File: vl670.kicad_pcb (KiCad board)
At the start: 4 copper layers, 60.3 x 22.4 mm, 72 parts, among them J1 Conn_01x07_Male, J2 USB_C_Receptacle, J3 Conn_01x07_Male, J4 USB3_A Receptacle, J5 Conn_01x02_Male, U1 HD3SS3220, U2 VL670, U3 4016, U4 TPS2061C-PXLI, U6 GD25D05, Y1 25MHz

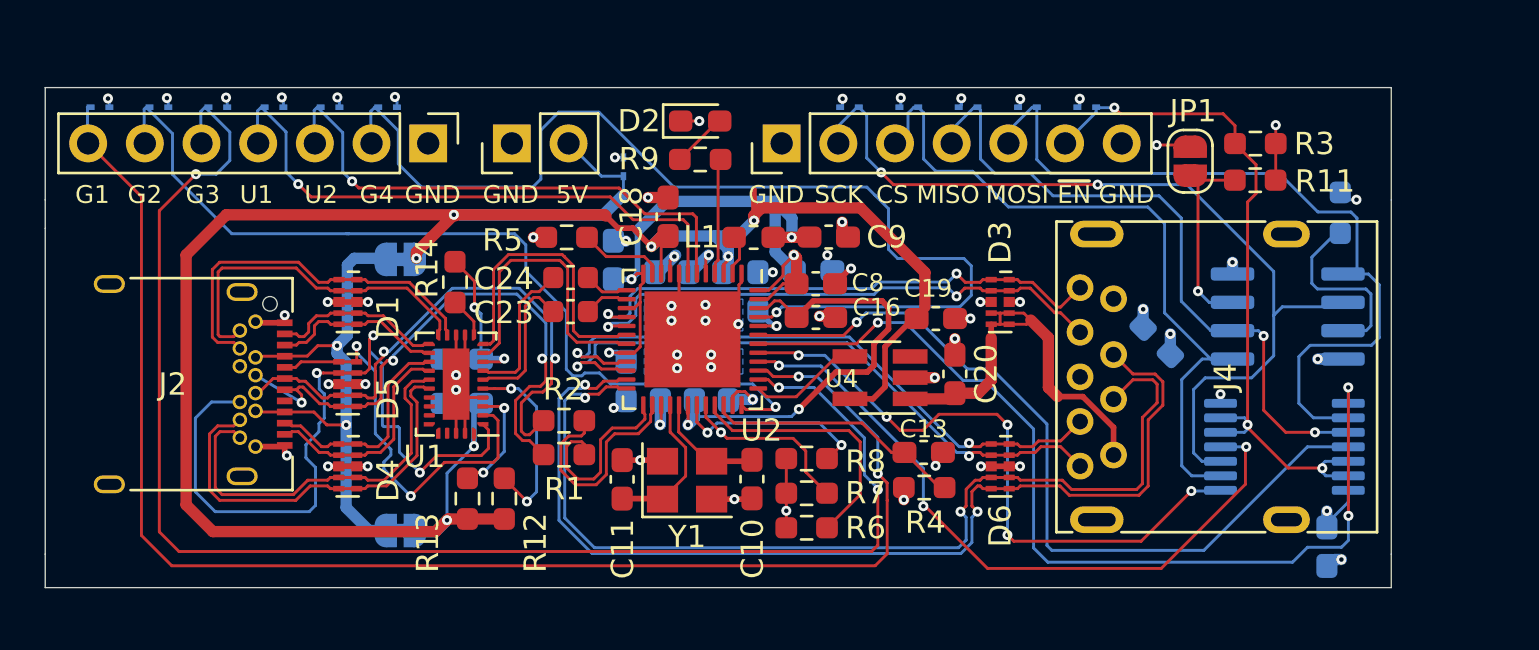
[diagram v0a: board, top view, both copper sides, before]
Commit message: First private release.
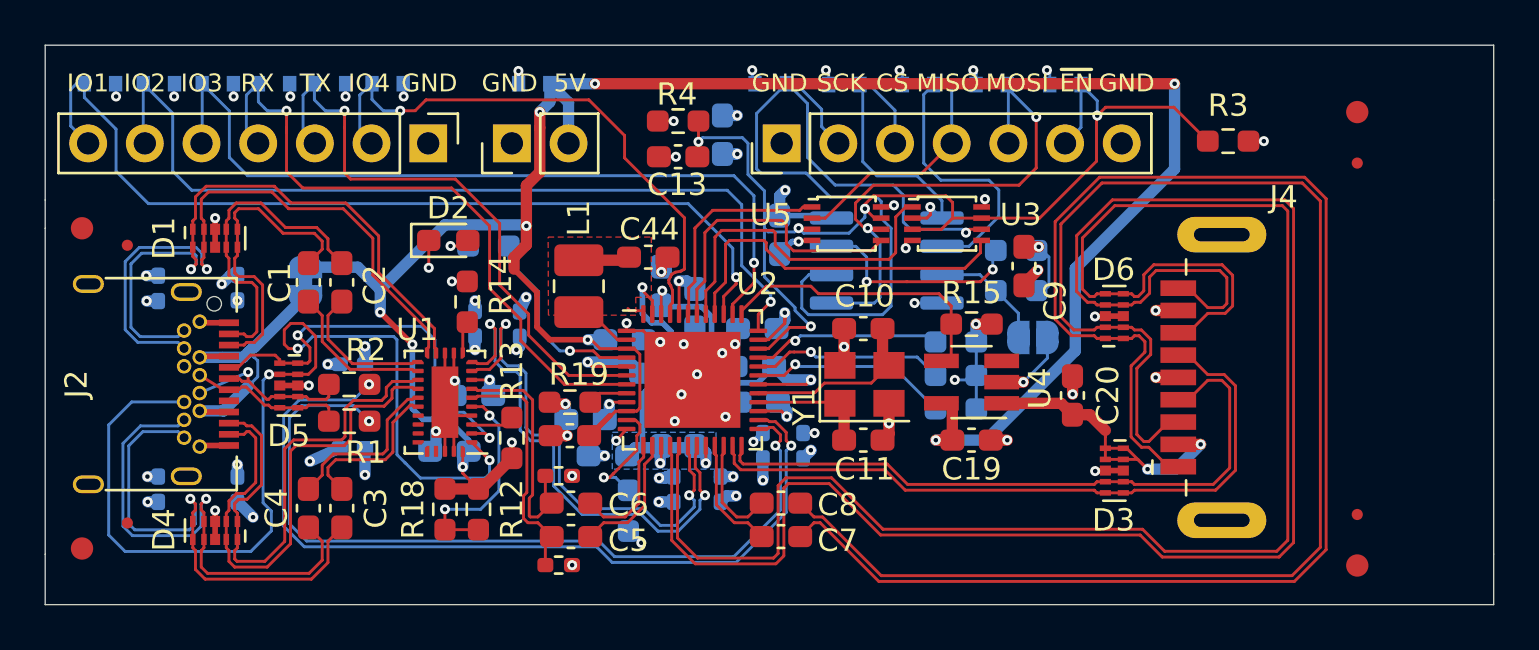
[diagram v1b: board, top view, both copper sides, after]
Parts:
- removed C14, C15, C16, C17, C18: 1uF, Capacitor_SMD:C_0603_1608Metric_Pad1.08x0.95mm_HandSolder
- removed C23, C24: 330nF, Capacitor_SMD:C_0603_1608Metric
- removed JP3: SolderJumper_2_Bridged, Jumper:SolderJumper-2_P1.3mm_Bridged_RoundedPad1.0x1.5mm
- added C31: 470nF, Capacitor_SMD:C_0603_1608Metric_Pad1.08x0.95mm_HandSolder, B.Cu at (199.7, 122.7)
- added C32: 470nF, Capacitor_SMD:C_0603_1608Metric_Pad1.08x0.95mm_HandSolder, B.Cu at (204.1, 124.0)
- added C33: 470nF, Capacitor_SMD:C_0603_1608Metric_Pad1.08x0.95mm_HandSolder, B.Cu at (204.0, 120.7)
- added C34: 470nF, Capacitor_SMD:C_0603_1608Metric_Pad1.08x0.95mm_HandSolder, B.Cu at (201.2, 119.8)
- added C35: 470nF, Capacitor_SMD:C_0603_1608Metric_Pad1.08x0.95mm_HandSolder, B.Cu at (196.3, 124.8)
- added C41: 1uF, Capacitor_SMD:C_0603_1608Metric_Pad1.08x0.95mm_HandSolder, B.Cu at (201.2, 125.1)
- added C42: 1uF, Capacitor_SMD:C_0603_1608Metric_Pad1.08x0.95mm_HandSolder, B.Cu at (197.3, 126.4)
- added C43: 1uF, Capacitor_SMD:C_0603_1608Metric_Pad1.08x0.95mm_HandSolder, B.Cu at (199.7, 125.1)
- added C44: 1uF, Capacitor_SMD:C_0603_1608Metric_Pad1.08x0.95mm_HandSolder, F.Cu at (199.1, 117.5)
- added C51: 1uF, Capacitor_SMD:C_0603_1608Metric_Pad1.08x0.95mm_HandSolder, F.Cu at (195.6, 125.5)
- added C52: 1uF, Capacitor_SMD:C_0603_1608Metric_Pad1.08x0.95mm_HandSolder, B.Cu at (198.1, 121.2)
- added C61: 1uF, Capacitor_SMD:C_0603_1608Metric_Pad1.08x0.95mm_HandSolder, B.Cu at (203.9, 122.4)
- added C62: 1uF, Capacitor_SMD:C_0603_1608Metric_Pad1.08x0.95mm_HandSolder, B.Cu at (199.7, 118.8)
- added C71: 470nF, Capacitor_SMD:C_0402_1005Metric_Pad0.74x0.62mm_HandSolder, B.Cu at (206.1, 126.0)
- added C72: 470nF, Capacitor_SMD:C_0402_1005Metric_Pad0.74x0.62mm_HandSolder, B.Cu at (204.2, 126.0)
- added C73: 470nF, Capacitor_SMD:C_0402_1005Metric_Pad0.74x0.62mm_HandSolder, B.Cu at (185.8, 122.3)
- added C74: 470nF, Capacitor_SMD:C_0402_1005Metric_Pad0.74x0.62mm_HandSolder, B.Cu at (185.8, 126.0)
- added C75: 470nF, Capacitor_SMD:C_0402_1005Metric_Pad0.74x0.62mm_HandSolder, B.Cu at (202.3, 127.9)
- added C76: 470nF, Capacitor_SMD:C_0402_1005Metric_Pad0.74x0.62mm_HandSolder, B.Cu at (200.2, 127.9)
- added C77: 470nF, Capacitor_SMD:C_0402_1005Metric_Pad0.74x0.62mm_HandSolder, B.Cu at (191.3, 120.5)
- added C78: 470nF, Capacitor_SMD:C_0402_1005Metric_Pad0.74x0.62mm_HandSolder, B.Cu at (193.3, 120.5)
- added C79: 470nF, Capacitor_SMD:C_0402_1005Metric_Pad0.74x0.62mm_HandSolder, B.Cu at (177.2, 118.9)
- added C80: 470nF, Capacitor_SMD:C_0402_1005Metric_Pad0.74x0.62mm_HandSolder, B.Cu at (180.7, 118.9)
- added C81: 470nF, Capacitor_SMD:C_0402_1005Metric_Pad0.74x0.62mm_HandSolder, B.Cu at (177.2, 127.9)
- added C82: 470nF, Capacitor_SMD:C_0402_1005Metric_Pad0.74x0.62mm_HandSolder, B.Cu at (180.7, 127.9)
- added FID1: Fiducial, vl670:StencilFiducial_1mm, F.Cu at (173.7, 116.2)
- added FID2: Fiducial, vl670:StencilFiducial_0.5mm, F.Cu at (175.8, 117.0)
- added FID3: Fiducial, vl670:StencilFiducial_1mm, F.Cu at (230.9, 111.0)
- added FID4: Fiducial, vl670:StencilFiducial_0.5mm, F.Cu at (175.8, 129.4)
- added FID5: Fiducial, vl670:StencilFiducial_1mm, F.Cu at (173.7, 130.6)
- added FID6: Fiducial, vl670:StencilFiducial_0.5mm, F.Cu at (230.9, 113.3)
- added FID7: Fiducial, vl670:StencilFiducial_1mm, F.Cu at (230.9, 131.3)
- added FID8: Fiducial, vl670:StencilFiducial_0.5mm, F.Cu at (230.9, 129.0)
- added R15: 10k, Resistor_SMD:R_0603_1608Metric_Pad0.98x0.95mm_HandSolder, F.Cu at (213.6, 120.5)
- added R16: 100K, Resistor_SMD:R_0402_1005Metric_Pad0.72x0.64mm_HandSolder, F.Cu at (195.1, 131.3)
- added R17: 100K, Resistor_SMD:R_0402_1005Metric_Pad0.72x0.64mm_HandSolder, F.Cu at (195.1, 127.3)
- added R18: 1.8M, Resistor_SMD:R_0603_1608Metric_Pad0.98x0.95mm_HandSolder, F.Cu at (190.0, 128.8)
- added R19: 0R, Resistor_SMD:R_0603_1608Metric_Pad0.98x0.95mm_HandSolder, F.Cu at (195.6, 124.0)
- added U5: 74LVC2G66, Package_SO:VSSOP-8_2.4x2.1mm_P0.5mm, F.Cu at (208.0, 116.0)
- C1, C3, C4, C5, C6, C7: value 1uF -> 220nF; moved to F.Cu
- C2: value 1uF -> 230nF; moved to F.Cu
- C22, C25, C26, C9: value 1uF -> 470nF
- C8: value 1uF -> 220nF
- D10, D11, D12, D13, D15, D16, D17, D18, D8, D9: value D_TVS -> ESD7951S; footprint Diode_SMD:D_SOD-923 -> Diode_SMD:D_SOD-523
- D14, D7: footprint Diode_SMD:D_SOD-923 -> Diode_SMD:D_SOD-523
- J2: footprint Connector_USB:USB_C_Receptacle_Amphenol_12401548E4-2A -> vl670:USB_C_Receptacle_XKB_U262-241N-4BV60
- J4: footprint Connector_USB:USB3_A_Molex_48393-001 -> vl670:USB3_A_Receptacle_Wuerth_692112030100_Horizontal
- JP1, R5, R6, R7, R8, R9: moved to B.Cu
- L1: footprint Inductor_SMD:L_0603_1608Metric_Pad1.05x0.95mm_HandSolder -> Inductor_SMD:L_1008_2520Metric_Pad1.43x2.20mm_HandSolder
- R10: value 10K -> 10k
- R11: value 10K -> 10k; moved to B.Cu
- R12: value 900k -> 1.8M
- U3: value 4016 -> 74LVC2G66; footprint Package_SO:TSSOP-14_4.4x5mm_P0.65mm -> Package_SO:VSSOP-8_2.4x2.1mm_P0.5mm; moved to F.Cu
- moved C22 32.8 mm to (202.4, 112.0), turned to 90 degrees
- moved C3 21.0 mm to (185.4, 128.8), turned to 270 degrees
- moved R4 19.8 mm to (200.4, 111.4)
- moved C4 19.6 mm to (183.9, 128.8)
- moved C1 19.3 mm to (183.9, 118.6)
- moved U6 18.1 mm to (209.8, 117.7), turned to 180 degrees
- moved U3 18.1 mm to (212.5, 116.0)
- moved C26 17.6 mm to (205.0, 116.5), turned to 270 degrees
- moved C13 17.2 mm to (200.4, 113.0), turned to 180 degrees
- moved C2 14.9 mm to (185.4, 118.6)
- moved R10 14.6 mm to (215.6, 117.2), turned to 180 degrees
- moved R5 12.6 mm to (198.2, 128.9), turned to 270 degrees
- moved D2 12.5 mm to (190.2, 116.8)
- moved JP2 11.9 mm to (183.8, 118.6), turned to 90 degrees
- moved R11 11.8 mm to (215.6, 119.0)
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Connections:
- net /D+ renamed /D_DEMUX+
- net /D- renamed /D_DEMUX-
- net /USB MUX/ESD/CC1 renamed /USB AC CAP/ESD/MUX/CC1
- net /USB MUX/ESD/CC2 renamed /USB AC CAP/ESD/MUX/CC2
- net /USB MUX/ESD/D+ renamed /USB AC CAP/ESD/MUX/D+
- net /USB MUX/ESD/D- renamed /USB AC CAP/ESD/MUX/D-
- net /USB MUX/ESD/RX2+ renamed /USB AC CAP/ESD/MUX/RX2+
- net /USB MUX/ESD/RX2- renamed /USB AC CAP/ESD/MUX/RX2-
- C1 pad 1: +3V3 -> /USB AC CAP/ESD/MUX/TX1_AC-
- C1 pad 2: GND -> /USB AC CAP/ESD/MUX/TX1-
- C13 pad 1: Net-(C13-Pad1) -> ~EXT_RESET
- C2 pad 1: +3V3 -> /USB AC CAP/ESD/MUX/TX1_AC+
- C2 pad 2: GND -> /USB AC CAP/ESD/MUX/TX1+
- C3 pad 1: +3V3 -> /USB AC CAP/ESD/MUX/TX2_AC-
- C3 pad 2: GND -> /USB AC CAP/ESD/MUX/TX2+
- C4 pad 1: +3V3 -> /USB AC CAP/ESD/MUX/TX2_AC+
- C4 pad 2: GND -> /USB AC CAP/ESD/MUX/TX2-
- C5 pad 1: +3V3 -> /SSTX_DEMUX-
- C5 pad 2: GND -> /USB AC CAP/ESD/MUX/TX_MUX_DC-
- C6 pad 1: +1V5 -> /SSTX_DEMUX+
- C6 pad 2: GND -> /USB AC CAP/ESD/MUX/TX_MUX_DC+
- C7 pad 1: +1V5 -> /DN_TX_AC-
- C7 pad 2: GND -> /DN_SSTX-
- C8 pad 1: +1V5 -> /DN_TX_AC+
- C8 pad 2: GND -> /DN_SSTX+
- C9 pad 1: +1V5 -> +3V3
- D1 pad 1: /USB MUX/ESD/RX1- -> /USB AC CAP/ESD/MUX/RX1+
- D1 pad 10: /USB MUX/ESD/RX1- -> /USB AC CAP/ESD/MUX/RX1+
- D1 pad 2: /USB MUX/ESD/RX1+ -> /USB AC CAP/ESD/MUX/RX1-
- D1 pad 4: /USB MUX/ESD/TX1+ -> /USB AC CAP/ESD/MUX/TX1+
- D1 pad 5: /USB MUX/ESD/TX1- -> /USB AC CAP/ESD/MUX/TX1-
- D1 pad 6: /USB MUX/ESD/TX1- -> /USB AC CAP/ESD/MUX/TX1-
- D1 pad 7: /USB MUX/ESD/TX1+ -> /USB AC CAP/ESD/MUX/TX1+
- D1 pad 9: /USB MUX/ESD/RX1+ -> /USB AC CAP/ESD/MUX/RX1-
- D17 pad 1: /eeprom/~ISP_ENABLE -> ~EXT_RESET
- D3 pad 1: /DN_USB3RX- -> +5V_SW
- D3 pad 10: /DN_USB3RX- -> +5V_SW
- D3 pad 2: /DN_USB3RX+ -> +5V_SW
- D3 pad 4: +5V_SW -> /DN_D-
- D3 pad 5: +5V_SW -> /DN_D+
- D3 pad 6: +5V_SW -> /DN_D+
- D3 pad 7: +5V_SW -> /DN_D-
- D3 pad 9: /DN_USB3RX+ -> +5V_SW
- D4 pad 4: /USB MUX/ESD/TX2+ -> /USB AC CAP/ESD/MUX/TX2-
- D4 pad 5: /USB MUX/ESD/TX2- -> /USB AC CAP/ESD/MUX/TX2+
- D4 pad 6: /USB MUX/ESD/TX2- -> /USB AC CAP/ESD/MUX/TX2+
- D4 pad 7: /USB MUX/ESD/TX2+ -> /USB AC CAP/ESD/MUX/TX2-
- D6 pad 1: /DN_USB3TX- -> /DN_TX_AC-
- D6 pad 10: /DN_USB3TX- -> /DN_TX_AC-
- D6 pad 2: /DN_USB3TX+ -> /DN_TX_AC+
- D6 pad 4: /DN_D- -> /DN_SSRX-
- D6 pad 5: /DN_D+ -> /DN_SSRX+
- D6 pad 6: /DN_D+ -> /DN_SSRX+
- D6 pad 7: /DN_D- -> /DN_SSRX-
- D6 pad 9: /DN_USB3TX+ -> /DN_TX_AC+
- J1 pad 6: /eeprom/~ISP_ENABLE -> ~EXT_RESET
- J2 pad A2: /USB MUX/ESD/TX1+ -> /USB AC CAP/ESD/MUX/TX1+
- J2 pad A3: /USB MUX/ESD/TX1- -> /USB AC CAP/ESD/MUX/TX1-
- J2 pad B10: /USB MUX/ESD/RX1- -> /USB AC CAP/ESD/MUX/RX1-
- J2 pad B11: /USB MUX/ESD/RX1+ -> /USB AC CAP/ESD/MUX/RX1+
- J2 pad B2: /USB MUX/ESD/TX2+ -> /USB AC CAP/ESD/MUX/TX2+
- J2 pad B3: /USB MUX/ESD/TX2- -> /USB AC CAP/ESD/MUX/TX2-
- J4 pad 5: /DN_USB3RX- -> /DN_SSRX-
- J4 pad 6: /DN_USB3RX+ -> /DN_SSRX+
- J4 pad 8: /DN_USB3TX- -> /DN_TX_AC+
- J4 pad 9: /DN_USB3TX+ -> /DN_TX_AC-
- R3 pad 2: /eeprom/~ISP_ENABLE -> ~EXT_RESET
- R4 pad 2: Net-(C13-Pad1) -> ~EXT_RESET
- U1 pad 10: /USB MUX/ESD/RX+ -> /SSRX_DEMUX+
- U1 pad 14: /USB MUX/ESD/RX1- -> /USB AC CAP/ESD/MUX/RX1+
- U1 pad 15: /USB MUX/ESD/RX1+ -> /USB AC CAP/ESD/MUX/RX1-
- U1 pad 16: /USB MUX/ESD/TX1+ -> /USB AC CAP/ESD/MUX/TX1_AC+
- U1 pad 17: /USB MUX/ESD/TX1- -> /USB AC CAP/ESD/MUX/TX1_AC-
- U1 pad 20: /USB MUX/ESD/TX2+ -> /USB AC CAP/ESD/MUX/TX2_AC+
- U1 pad 21: /USB MUX/ESD/TX2- -> /USB AC CAP/ESD/MUX/TX2_AC-
- U1 pad 6: /USB MUX/ESD/TX- -> /USB AC CAP/ESD/MUX/TX_MUX_DC-
- U1 pad 7: /USB MUX/ESD/TX+ -> /USB AC CAP/ESD/MUX/TX_MUX_DC+
- U1 pad 9: /USB MUX/ESD/RX- -> /SSRX_DEMUX-
- U2 pad 13: /TX+ -> /SSTX_DEMUX+
- U2 pad 14: /TX- -> /SSTX_DEMUX-
- U2 pad 16: /DN_USB3RX- -> /DN_SSRX-
- U2 pad 17: /DN_USB3RX+ -> /DN_SSRX+
- U2 pad 18: /USB MUX/ESD/RX+ -> /SSRX_DEMUX-
- U2 pad 19: /USB MUX/ESD/RX- -> /SSRX_DEMUX+
- U2 pad 21: /DN_USB3TX- -> /DN_SSTX-
- U2 pad 22: /DN_USB3TX+ -> /DN_SSTX+
- U2 pad 34: Net-(C13-Pad1) -> ~EXT_RESET
- U2 pad 8: GND -> Net-(R19-Pad1)
- U3 pad 3: /eeprom/ISP_SCK -> ~EXT_RESET
- U3 pad 4: /eeprom/SCK -> GND
- U3 pad 5: /eeprom/~ISP_ENABLE -> /eeprom/SCK
- U3 pad 6: /eeprom/~ISP_ENABLE -> /eeprom/ISP_SCK
- U3 pad 7: GND -> ~EXT_RESET
- U3 pad 8: /eeprom/MOSI -> +3V3
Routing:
- net /DN_SSRX-: track 0.00 -> 78.7 mm
- net /DN_SSRX+: track 0.00 -> 76.7 mm
- net /DN_TX_AC-: track 0.00 -> 71.4 mm
- net /DN_TX_AC+: track 0.00 -> 69.5 mm
- net ~EXT_RESET: track 0.00 -> 50.9 mm, vias 0 -> 5
- net /eeprom/~ISP_ENABLE: track 33.4 -> 0.00 mm, vias 3 -> 0
- net Net-(D9-Pad1): track 66.6 -> 36.8 mm, vias 3 -> 1
- net /eeprom/MOSI: track 42.4 -> 13.2 mm, vias 3 -> 0
- net /USB AC CAP/ESD/MUX/RX1-: track 0.00 -> 28.9 mm, vias 0 -> 1
- net /DN_USB3TX+: track 28.7 -> 0.00 mm, vias 2 -> 0
- net /DN_USB3TX-: track 28.7 -> 0.00 mm, vias 2 -> 0
- net /D_DEMUX+: track 10.1 -> 38.7 mm, vias 0 -> 2
- net /USB AC CAP/ESD/MUX/RX1+: track 0.00 -> 28.5 mm, vias 0 -> 1
- net /D_DEMUX-: track 8.69 -> 37.1 mm, vias 0 -> 2
- net /eeprom/MISO: track 36.6 -> 9.62 mm, vias 1 -> 0
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- added copper zone on B.Cu, net +1V5
- added copper zone on F.Cu, net +1V5
- removed copper zone on B.Cu, net GND
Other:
- board size 60.3 x 22.4 mm -> 64.9 x 25.1 mm
- board text added: "IO1"
- board text added: "IO2"
- board text added: "IO3"
- board text added: "IO4"
- board text added: "RX"
- board text added: "TX"
- board text removed: "G1"
- board text removed: "G2"
- board text removed: "G3"
- board text removed: "G4"
- board text removed: "U1"
- board text removed: "U2"
